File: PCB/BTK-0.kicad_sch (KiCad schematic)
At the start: 95 parts, among them J1 USB_C_Receptacle_USB2.0_16P, J2 BAT+, J3 BAT-, J6 Conn_01x16_Pin, J7 Conn_01x16_Socket, SW1 EN, SW10 1,2, SW11 2,2, SW12 3,2, SW13 4,2, SW14 5,2, SW15 6,2, SW16 1,3, SW17 2,3, SW18 3,3, SW19 4,3, SW2 BOOT, SW20 5,3, SW21 6,3, SW22 1,4, SW23 2,4, SW24 3,4, SW25 4,4, SW26 5,4, SW27 6,4, SW28 1,4, SW29 2,4, SW3 RotaryEncoder_Switch_MP, SW30 3,4, SW31 4,4, SW32 5,4, SW33 6,4, SW4 1,1, SW5 2,1, SW6 3,1, SW7 4,1, SW8 5,1, SW9 6,1, U1 NCP1117-3.3_SOT223, U2 NCP1117-3.3_SOT223, U3 USBLC6-2SC6, U4 ESP32-C6-MINI-1, U5 TVS1400DRV

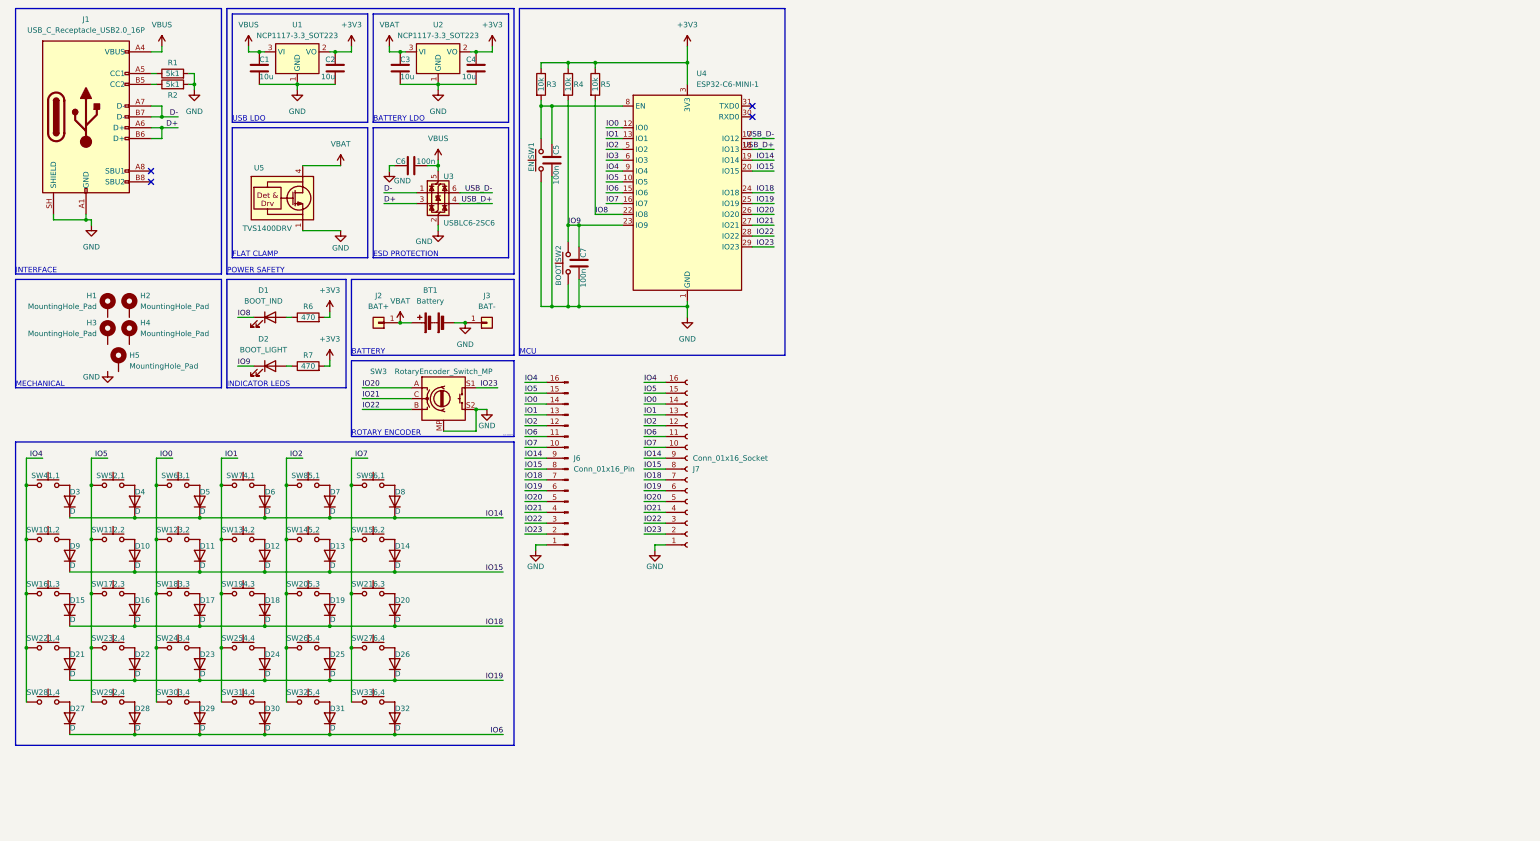
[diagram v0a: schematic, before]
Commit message: im boutta die son
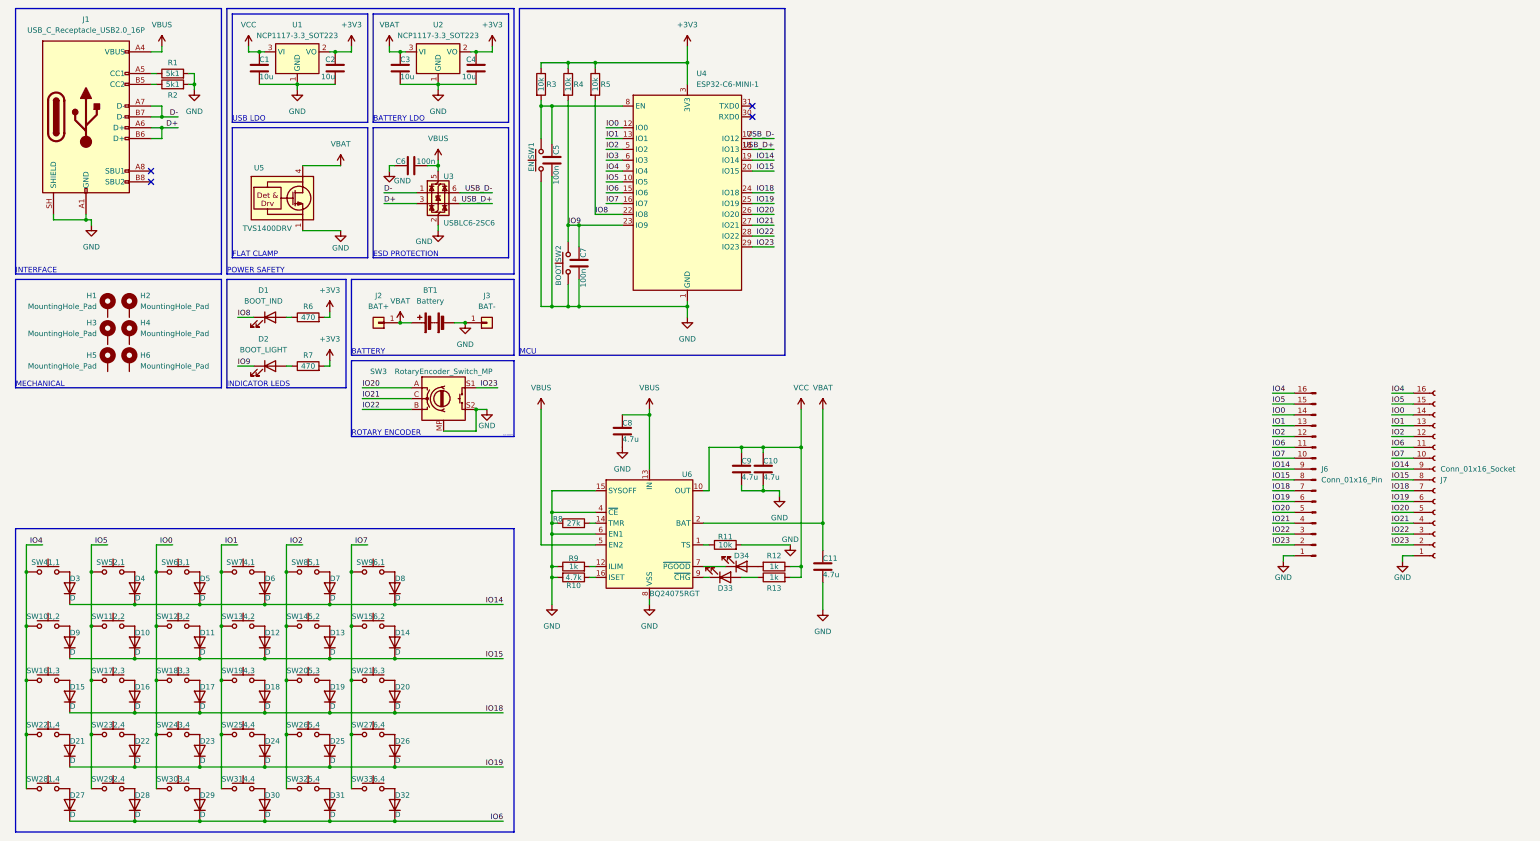
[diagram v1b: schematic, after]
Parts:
- added C10, C11, C8, C9: 4.7u, Capacitor_SMD:C_0402_1005Metric, symbol Device:C
- added D33, D34: LED, LED_SMD:LED_0805_2012Metric, symbol Device:LED
- added H6: MountingHole_Pad, MountingHole:MountingHole_3.2mm_M3_ISO7380, symbol Mechanical:MountingHole_Pad
- added R10: 4.7k, Resistor_SMD:R_0402_1005Metric, symbol Device:R
- added R11: 10k, Resistor_SMD:R_0402_1005Metric, symbol Device:R
- added R12, R13, R9: 1k, Resistor_SMD:R_0402_1005Metric, symbol Device:R
- added R8: 27k, Resistor_SMD:R_0402_1005Metric, symbol Device:R
- added U6: BQ24075RGT, Package_DFN_QFN:VQFN-16-1EP_3x3mm_P0.5mm_EP1.6x1.6mm, symbol Battery_Management:BQ24075RGT
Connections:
- net GND: now also C10.2, C11.2, C8.2, C9.2, R10.2, R11.2, R8.1, R9.1, U6.15 (SYSOFF), U6.17 (VSS), U6.4 (~{CE}), U6.6 (EN1), U6.8 (VSS)
- net VBAT: now also C11.1, U6.2 (BAT), U6.3 (BAT)
- net VBUS: now also C8.1, U6.13 (IN), U6.5 (EN2); no longer C1.1, U1.3 (VI)
- new net: R11.1, U6.1 (TS)
- new net: R9.2, U6.12 (ILIM)
- new net: R8.2, U6.14 (TMR)
- new net: R10.1, U6.16 (ISET)
- new net: D34.1 (K), U6.7 (~{PGOOD})
- new net: D33.1 (K), U6.9 (~{CHG})
- new net: D33.2 (A), R13.1
- new net: D34.2 (A), R12.2
- new net VCC: C1.1, C10.1, C9.1, R12.1, R13.2, U1.3 (VI), U6.10 (OUT), U6.11 (OUT)
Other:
- moved on the sheet: D10, D11, D12, D13, D14, D15, D16, D17, D18, D19, D20, D21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
